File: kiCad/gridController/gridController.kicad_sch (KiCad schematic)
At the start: 9 parts

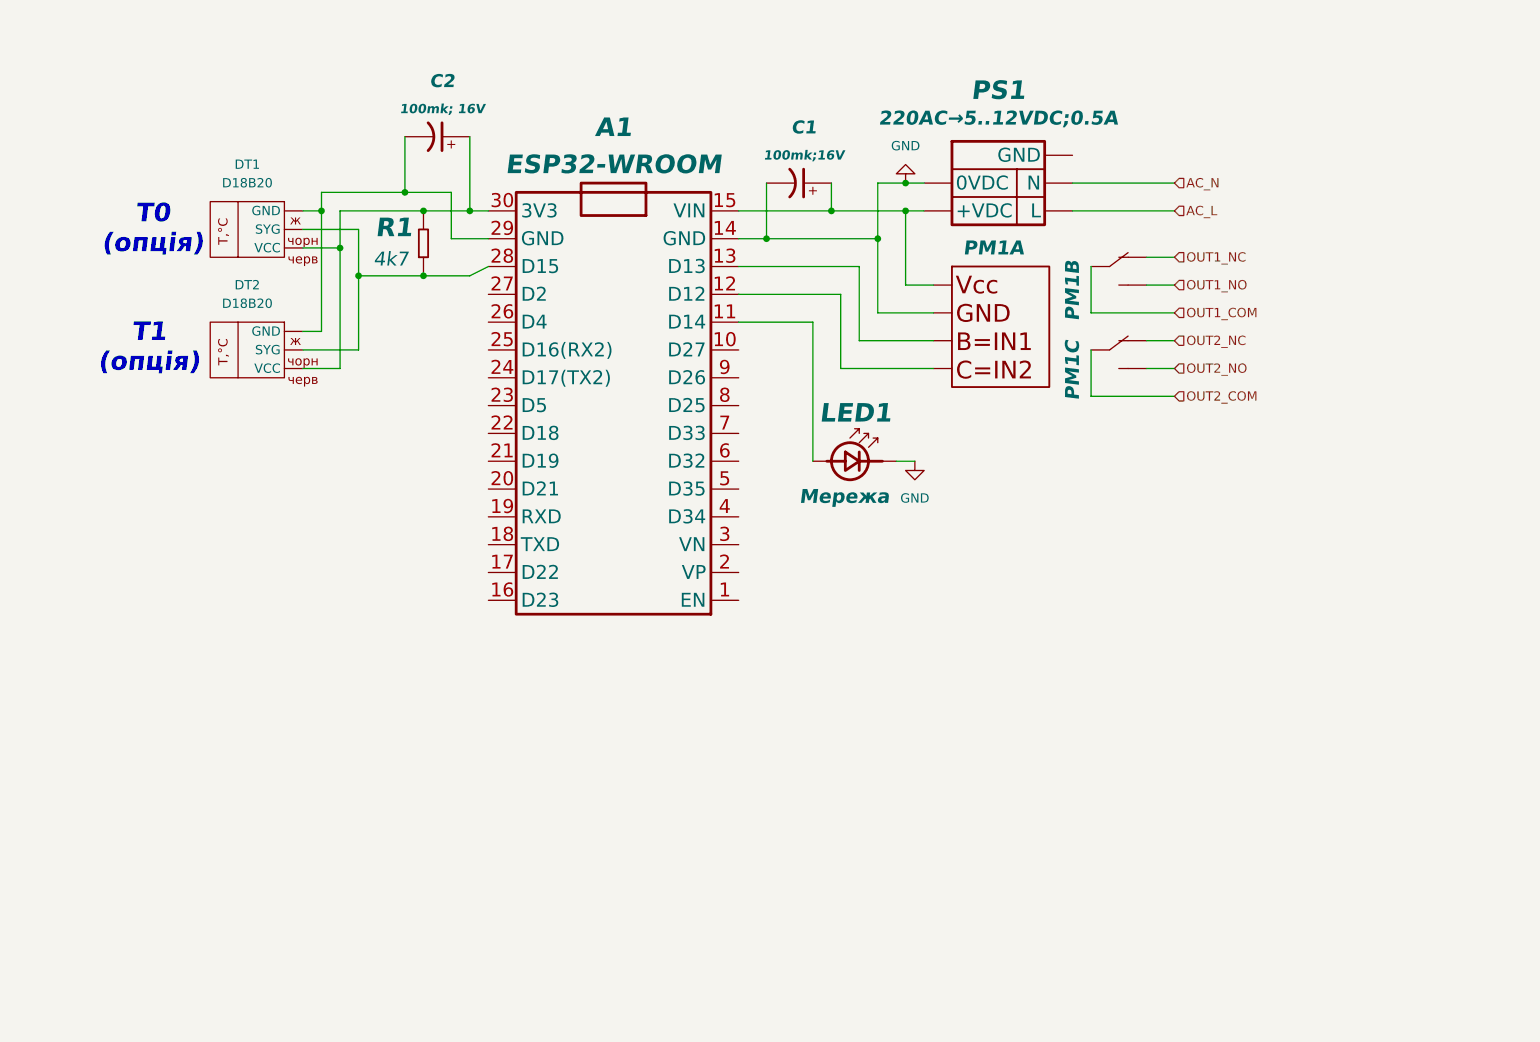
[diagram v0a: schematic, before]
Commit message: 2026-01-30 Was added CORS requests
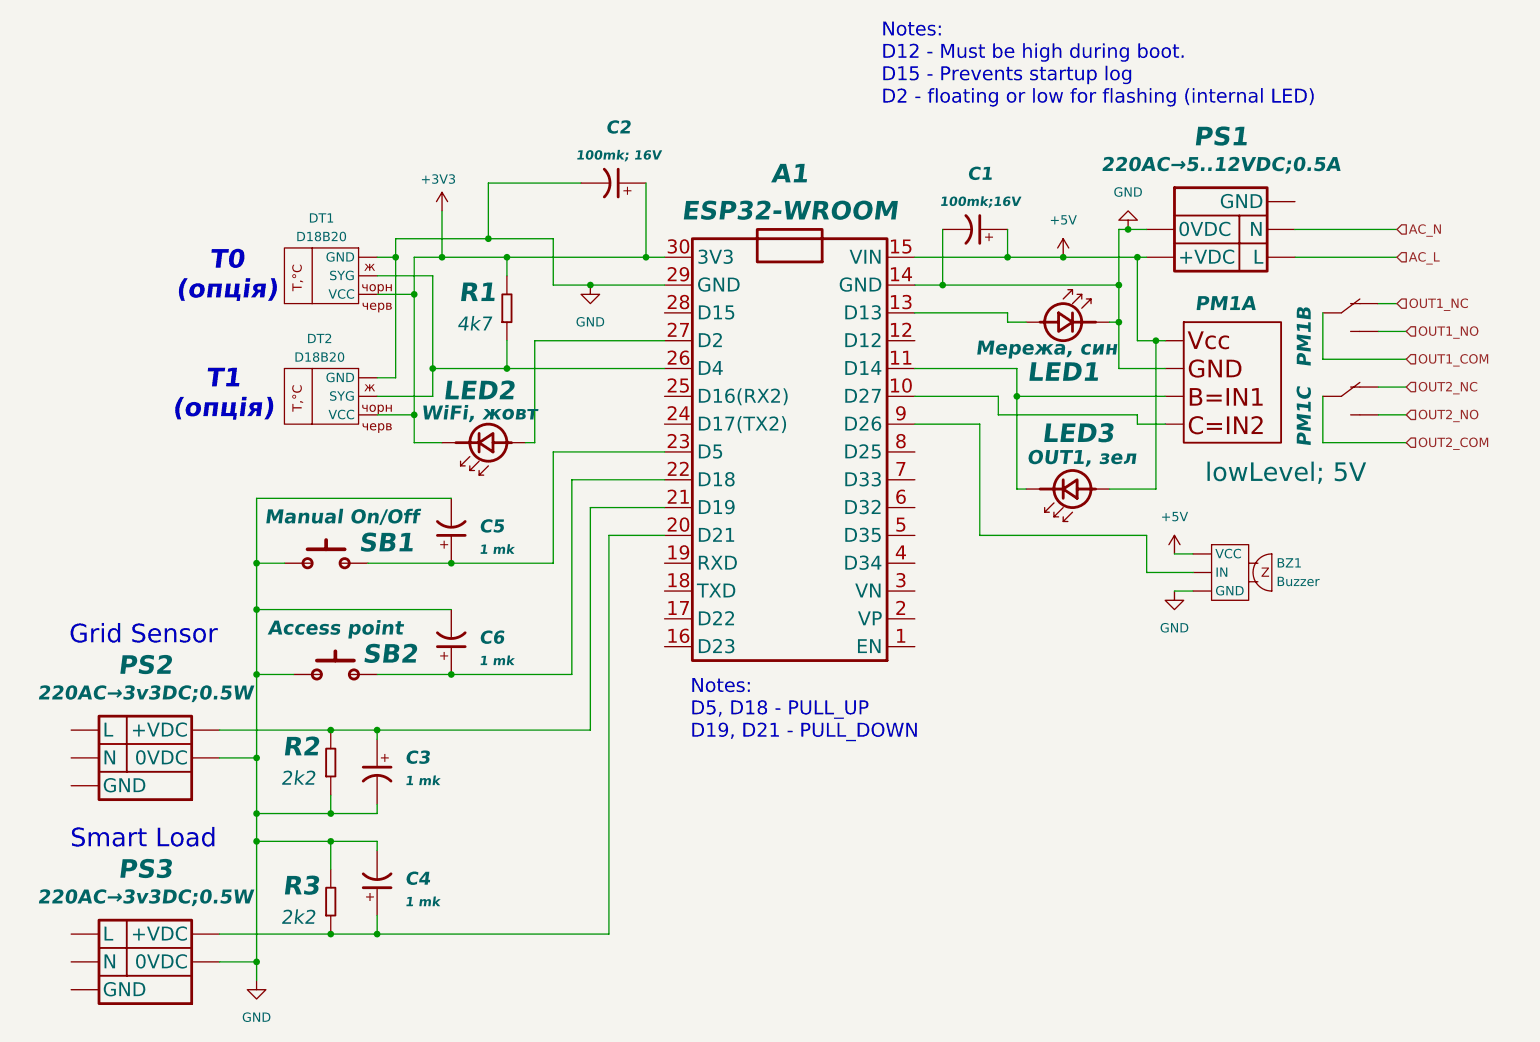
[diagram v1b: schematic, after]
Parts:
- added BZ1: Buzzer, symbol B_Electronics:T_Buzzer_Active
- added C3, C4, C5, C6: 1 mk, symbol B_Electronics:Конденсатор_Електроліт
- added LED2: WiFi, жовт, symbol B_Electronics:LED
- added LED3: OUT1, зел, symbol B_Electronics:LED
- added PS2, PS3: 220АС→3v3DC;0.5W, symbol B_Electronics:БЖ_AC-DC
- added R2, R3: 2k2, symbol B_Electronics:Резистор
- added SB1, SB2: Кнопка S2PR-P1K, чорна, д22, symbol B_EL_General:Кнопка_NO
- LED1: value Мережа -> Мережа, син
- PM1: value ~ -> lowLevel; 5V; Склад Модуль реле, DC5V, 2 канали; lowHighLevel -> Модуль реле, DC5V, 2 канали; lowLevel(!)
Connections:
- net GND: now also A1.29 (GND), C2.1, DT1.3 (GND), DT2.3 (GND), BZ1.3 (GND), C3.1, C4.1, C5.1, C6.1, PS2.4 (0VDC), PS3.4 (0VDC), R2.1, R3.2, SB1.1, SB2.1
- net at PM1.1 (IN1): now also A1.11 (D14), LED3.2 (-); no longer A1.13 (D13)
- net at PM1.2 (IN2): now also A1.10 (D27); no longer A1.12 (D12)
- net +5V: now reaches A1.15 (VIN), C1.2, PM1.3 (VCC), PS1.3 (+VDC)
- net +5V: now also BZ1.1 (VCC), LED3.1 (+)
- net +3V3: now reaches A1.30 (3V3), C2.2, DT1.1 (VCC), DT2.1 (VCC), R1.2
- net +3V3: now also LED2.2 (-)
- net at DT1.2 (SYG), DT2.2 (SYG), R1.1: now also A1.26 (D4); no longer A1.28 (D15)
- net at LED1.1 (+): now also A1.13 (D13); no longer A1.11 (D14)
- net at A1.20 (D21): now also C4.2, PS3.3 (+VDC), R3.1
- net at A1.21 (D19): now also C3.2, PS2.3 (+VDC), R2.2
- net at A1.22 (D18): now also C6.2, SB2.2
- net at A1.23 (D5): now also C5.2, SB1.2
- net at A1.27 (D2): now also LED2.1 (+)
- net at A1.9 (D26): now also BZ1.2 (IN)
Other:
- note added: "Grid Sensor"
- note added: "Notes: D12 - Must be high during boot. D15 - Prevents startup log D2 - floating or low for flashing (internal LED)"
- note added: "Notes: D5, D18 - PULL_UP D19, D21 - PULL_DOWN"
- note added: "Smart Load"
- moved on the sheet: A1, C1, C2, DT1, DT2, LED1, PM1A, PM1B, PM1C, PS1, R1
